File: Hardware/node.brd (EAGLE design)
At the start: 100 x 80 mm, 47 parts, among them J1 USB_B, M1 SERVO, M2 SERVO, Q1 16MHz, U1 MAX3485CSA

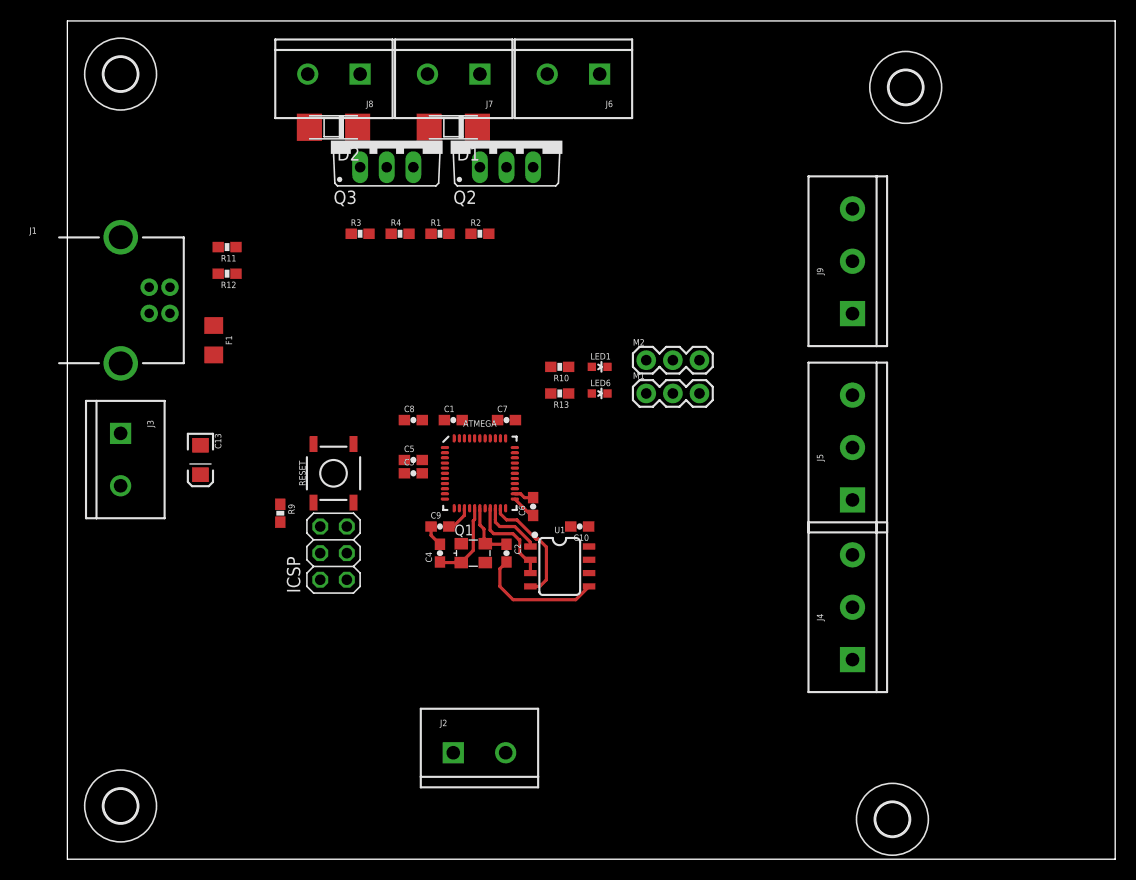
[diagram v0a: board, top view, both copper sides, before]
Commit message: Hardware pcb design
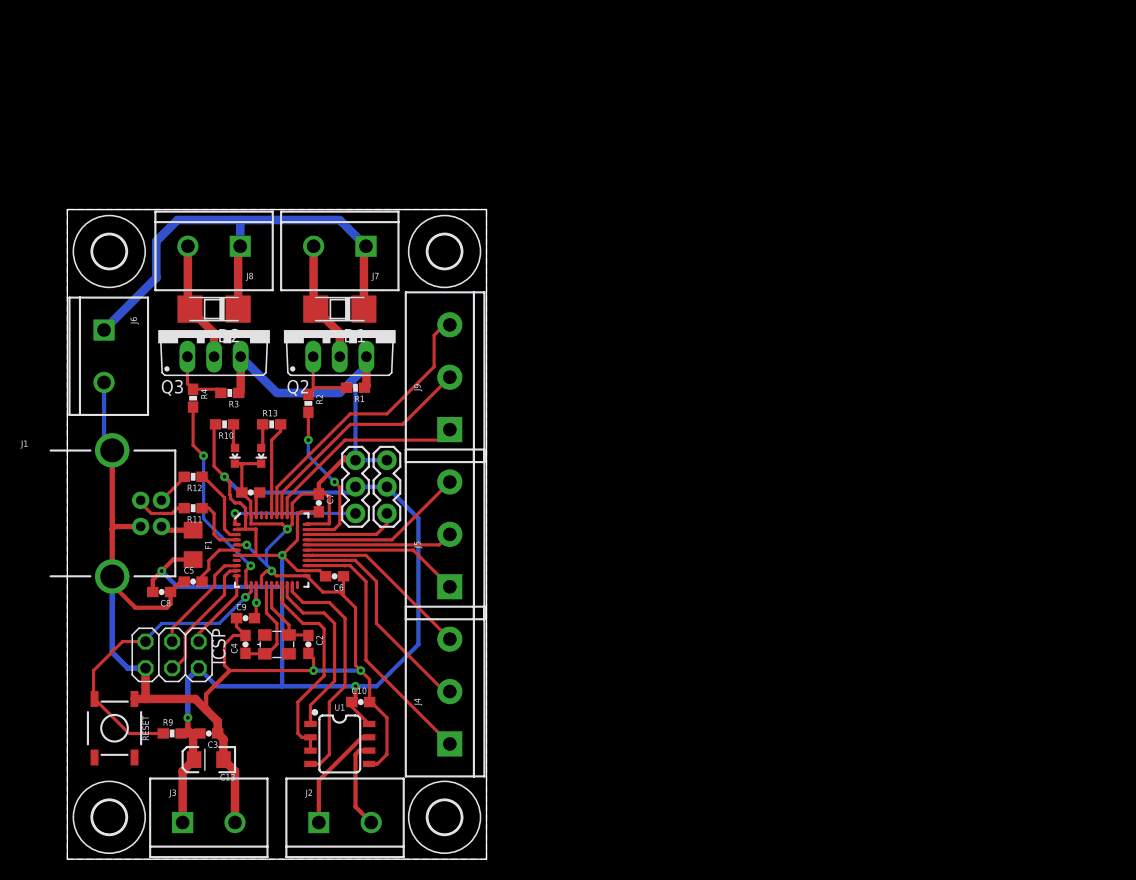
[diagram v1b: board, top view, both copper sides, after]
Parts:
- moved J6 53.2 mm to (3.50, 50.5), turned to 270 degrees
- moved H2 46.7 mm to (36.0, 58.0)
- moved H3 42.7 mm to (36.0, 4.00)
- moved J9 40.0 mm to (36.5, 41.0)
- moved J5 39.3 mm to (36.5, 26.0)
- moved J4 39.3 mm to (36.5, 11.0)
- moved J3 37.6 mm to (11.0, 3.50), turned to 0 degrees
- moved LED1 35.8 mm to (16.0, 38.5), turned to 180 degrees
- moved LED6 32.8 mm to (18.5, 38.5), turned to 180 degrees
- moved R10 32.5 mm to (15.0, 41.5)
- moved RESET 32.1 mm to (4.50, 12.5), turned to 270 degrees
- moved C3 31.6 mm to (13.5, 12.0), turned to 180 degrees
- moved M2 31.4 mm to (27.5, 33.0), turned to 90 degrees
- moved C8 29.1 mm to (9.00, 25.5), turned to 180 degrees
- moved C13 28.6 mm to (13.5, 9.50), turned to 180 degrees
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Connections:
- removed net D14: ATMEGA.8
- net A3: now also R13.2
- net D10: now also J5.3; no longer J4.1
- net D12: now also J4.2; no longer R13.2
- net D3: no longer J4.2
- net D4: now also J4.1; no longer J4.3
- net D5: now also M1.1; no longer J5.1
- net D6: now also J4.3; no longer J5.2
- net D7: now also M2.1; no longer J5.3
- net D8: now also J5.1; no longer M1.1
- net D9: now also J5.2; no longer M2.1
- net GND: now also J3.2; no longer J3.1
- net VCC: now also J3.1; no longer J3.2
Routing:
- net GND: track 16.6 -> 193.2 mm, vias 0 -> 5
- net VCC: track 4.50 -> 145.8 mm, vias 0 -> 6
- net +12V: track 0.00 -> 47.1 mm
- net RESET: track 0.00 -> 29.6 mm, vias 0 -> 1
- net A2: track 0.00 -> 27.3 mm
- net D4: track 0.00 -> 25.1 mm
- net A1: track 0.00 -> 22.7 mm
- net D12: track 0.00 -> 21.2 mm
- net A0: track 0.00 -> 19.9 mm
- net D11: track 0.00 -> 19.5 mm, vias 0 -> 2
- net D6: track 0.00 -> 17.0 mm
- net D10: track 0.00 -> 16.0 mm
- net D13: track 0.00 -> 15.3 mm, vias 0 -> 2
- net D8: track 0.00 -> 15.1 mm
- net D9: track 0.00 -> 14.1 mm
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- added copper zone on layer 1, net GND
- added copper zone on layer 16, net GND
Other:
- board size 100 x 80 mm -> 40 x 62 mm
